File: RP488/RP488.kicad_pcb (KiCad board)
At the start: 2 copper layers, 56.1 x 53.1 mm, 25 parts, among them J1 GPIB, J2 Test, U1 SN75160, U2 SN75161, U3 SN74LV245ATDW

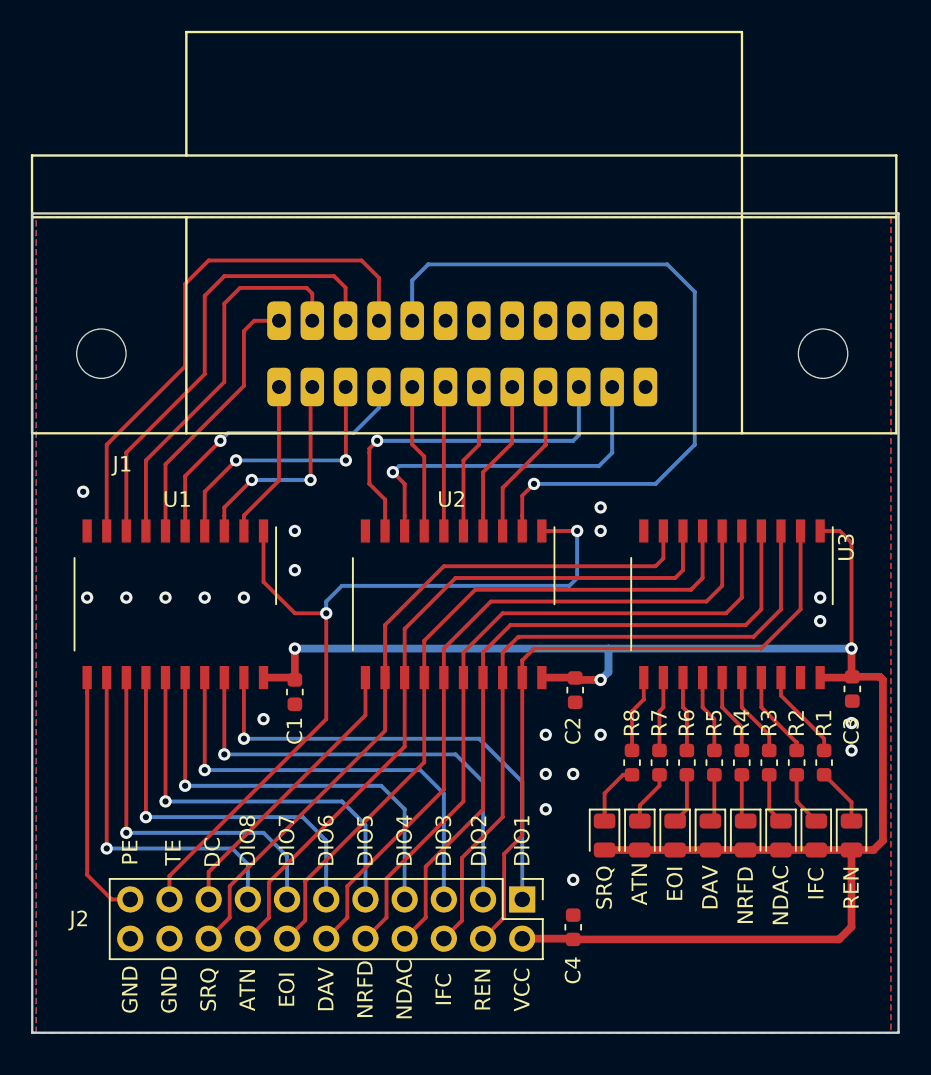
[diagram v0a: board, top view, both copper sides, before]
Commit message: SWD connector and schematic changes
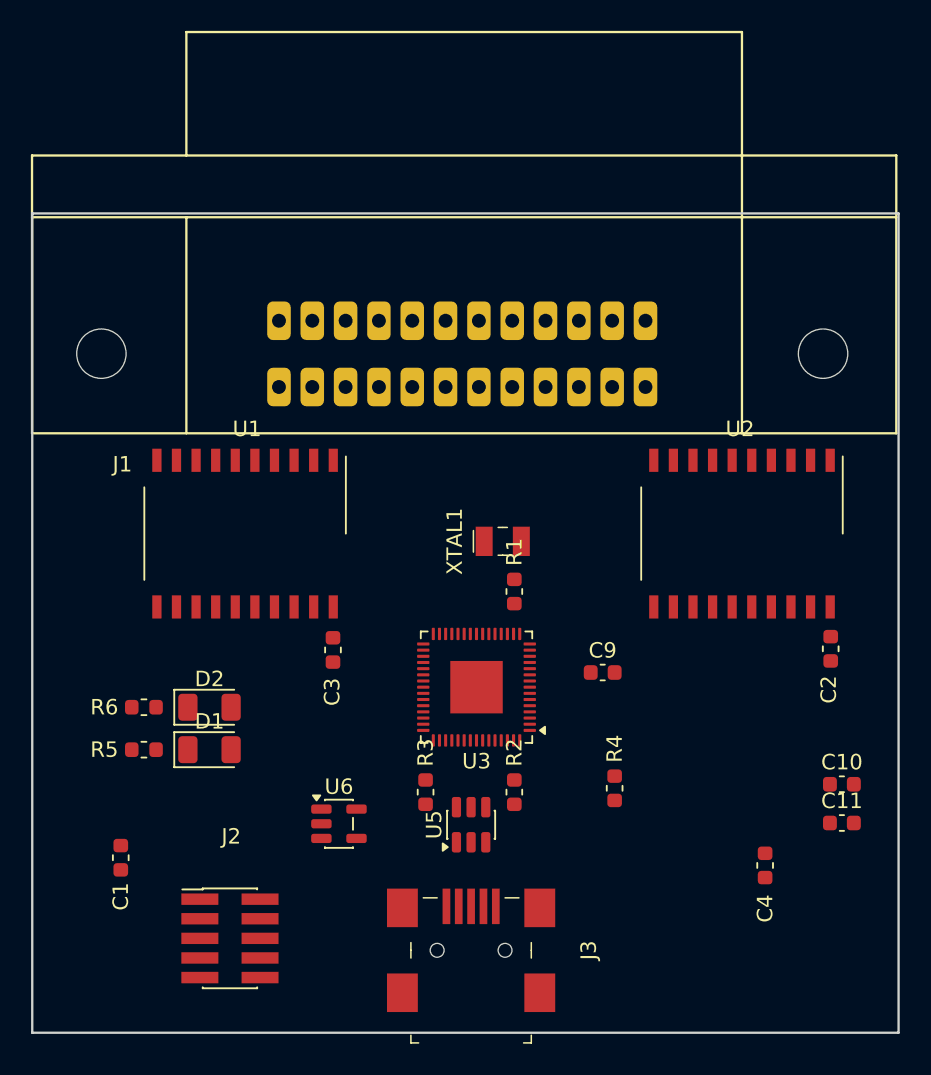
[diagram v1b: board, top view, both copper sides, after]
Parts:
- removed D3, D4, D5, D6, D7, D8: LED, LED_SMD:LED_0805_2012Metric
- removed R7, R8: 330R, Resistor_SMD:R_0603_1608Metric
- added C10: 100n, Capacitor_SMD:C_0603_1608Metric, F.Cu at (164.5, 100.7)
- added C11: 100n, Capacitor_SMD:C_0603_1608Metric, F.Cu at (164.5, 103.2)
- added C9: 100n, Capacitor_SMD:C_0603_1608Metric, F.Cu at (149.0, 93.5)
- added J3: USB Mini, GPIB:USB_Mini_B_Female_690-005-299-043, F.Cu at (140.4, 111.5)
- added U5: USBLC6-2SC6, Package_TO_SOT_SMD:SOT-23-6, F.Cu at (140.4, 103.4)
- added U6: LD3985M33R_SOT23, Package_TO_SOT_SMD:SOT-23-5, F.Cu at (131.9, 103.3)
- added XTAL1: 12MHz, GPIB:SMD-2_3.2x1.5mm, F.Cu at (142.5, 85.0)
- D1, D2: footprint LED_SMD:LED_0805_2012Metric -> LED_SMD:LED_1206_3216Metric
- J2: value Test -> SWD; footprint Connector_PinHeader_2.54mm:PinHeader_2x11_P2.54mm_Vertical -> GPIB:PinHeader_2x05_P1.27mm_Vertical_SMD
- R1, R5, R6: value 330R -> 1K
- R2, R3: value 330R -> 27R
- R4: value 330R -> 33R
- U3: value SN74LV245ATDW -> RP2354A; footprint Package_SO:SO-20_12.8x7.5mm_P1.27mm -> Package_DFN_QFN:QFN-60-1EP_7x7mm_P0.4mm_EP3.4x3.4mm
- moved D1 42.0 mm to (123.5, 98.5), turned to 0 degrees
- moved D2 40.2 mm to (123.5, 95.8), turned to 0 degrees
- moved R5 37.0 mm to (119.2, 98.5), turned to 180 degrees
- moved R6 35.4 mm to (119.2, 95.8), turned to 180 degrees
- moved C3 33.7 mm to (131.5, 92.0)
- moved R1 22.9 mm to (143.2, 88.2)
- moved R3 22.3 mm to (137.5, 101.2)
- moved U2 19.2 mm to (158.0, 84.5)
- moved J2 19.1 mm to (124.8, 110.7), turned to 0 degrees
- moved R2 18.4 mm to (143.2, 101.2)
- moved U3 17.4 mm to (140.8, 94.5), turned to 180 degrees
- moved C2 16.8 mm to (163.8, 92.0)
- moved C1 15.6 mm to (117.8, 105.5)
- moved C4 13.1 mm to (159.5, 106.0)
- moved R4 8.40 mm to (149.8, 101.0)
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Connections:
- D1 pad 1: Net-(D1-Pad1) -> Net-(D1-K)
- D1 pad 2: +5V -> Net-(D1-A)
- D2 pad 1: Net-(D2-Pad1) -> Net-(D2-K)
- D2 pad 2: +5V -> Net-(D2-A)
- J1 pad 12: Net-(J1-Pad12) -> unconnected-(J1-Pin_12-Pad12)
- J2 pad 1: Net-(J2-Pad1) -> +3V3
- J2 pad 10: Net-(J2-Pad10) -> /nRESET
- J2 pad 2: +5V -> /SWDIO
- J2 pad 3: Net-(J2-Pad3) -> GNDD
- J2 pad 4: Net-(J2-Pad4) -> /SWDCLK
- J2 pad 5: Net-(J2-Pad5) -> GNDD
- J2 pad 6: Net-(J2-Pad6) -> /SWO
- J2 pad 7: Net-(J2-Pad7) -> unconnected-(J2-Pin_7-Pad7)
- J2 pad 8: Net-(J2-Pad8) -> /TDI
- J2 pad 9: Net-(J2-Pad9) -> unconnected-(J2-Pin_9-Pad9)
- R1 pad 1: Net-(D1-Pad1) -> Net-(C5-Pad1)
- R1 pad 2: Net-(R1-Pad2) -> Net-(U3-XOUT)
- R2 pad 1: Net-(D2-Pad1) -> Net-(R2-Pad1)
- R2 pad 2: Net-(R2-Pad2) -> Net-(U3-USB_DP)
- R3 pad 2: Net-(R3-Pad2) -> Net-(U3-USB_DM)
- R4 pad 1: Net-(D4-Pad1) -> Net-(U3-VREG_AVDD)
- R4 pad 2: Net-(R4-Pad2) -> +3V3
- R5 pad 1: Net-(D5-Pad1) -> Net-(D1-K)
- R5 pad 2: Net-(R5-Pad2) -> GNDD
- R6 pad 1: Net-(D6-Pad1) -> Net-(D2-K)
- R6 pad 2: Net-(R6-Pad2) -> GNDD
- U1 pad 1: Net-(J2-Pad19) -> Net-(U1-TE)
- U1 pad 11: Net-(J2-Pad21) -> Net-(U1-PE)
- U1 pad 12: Net-(J2-Pad15) -> Net-(U1-D8)
- U1 pad 13: Net-(J2-Pad13) -> Net-(U1-D7)
- U1 pad 14: Net-(J2-Pad11) -> Net-(U1-D6)
- U1 pad 15: Net-(J2-Pad9) -> Net-(U1-D5)
- U1 pad 16: Net-(J2-Pad7) -> Net-(U1-D4)
- U1 pad 17: Net-(J2-Pad5) -> Net-(U1-D3)
- U1 pad 18: Net-(J2-Pad3) -> Net-(U1-D2)
- U1 pad 19: Net-(J2-Pad1) -> Net-(U1-D1)
- U1 pad 9: /DIO8 -> unconnected-(U1-B8-Pad9)
- U2 pad 1: Net-(J2-Pad19) -> Net-(U1-TE)
- U2 pad 11: Net-(J2-Pad17) -> Net-(U2-DC)
- U2 pad 12: Net-(J2-Pad18) -> Net-(U3-GPIO13)
- U2 pad 13: Net-(J2-Pad16) -> Net-(U3-GPIO12)
- U2 pad 14: Net-(J2-Pad14) -> Net-(U3-GPIO11)
- U2 pad 15: Net-(J2-Pad12) -> Net-(U3-GPIO8)
- U2 pad 16: Net-(J2-Pad10) -> Net-(U3-GPIO9)
- U2 pad 17: Net-(J2-Pad8) -> Net-(U3-GPIO10)
- U2 pad 18: Net-(J2-Pad6) -> Net-(U3-GPIO14)
- U2 pad 19: Net-(J2-Pad4) -> Net-(U3-GPIO15)
- U3 pad 1: +5V -> +3V3
- U3 pad 10: GNDD -> Net-(U1-D8)
- U3 pad 11: Net-(R8-Pad2) -> +3V3
- U3 pad 12: Net-(R7-Pad2) -> Net-(U3-GPIO8)
- U3 pad 13: Net-(R6-Pad2) -> Net-(U3-GPIO9)
- U3 pad 14: Net-(R5-Pad2) -> Net-(U3-GPIO10)
- U3 pad 15: Net-(R4-Pad2) -> Net-(U3-GPIO11)
- U3 pad 16: Net-(R3-Pad2) -> Net-(U3-GPIO12)
- U3 pad 17: Net-(R2-Pad2) -> Net-(U3-GPIO13)
- U3 pad 18: Net-(R1-Pad2) -> Net-(U3-GPIO14)
- U3 pad 19: GNDD -> Net-(U3-GPIO15)
- U3 pad 2: Net-(J2-Pad4) -> Net-(U1-D1)
- U3 pad 20: +5V -> +3V3
- U3 pad 3: Net-(J2-Pad6) -> Net-(U1-D2)
- U3 pad 4: Net-(J2-Pad8) -> Net-(U1-D3)
- U3 pad 5: Net-(J2-Pad10) -> Net-(U1-D4)
- U3 pad 6: Net-(J2-Pad12) -> Net-(U3-VREG_FB)
- U3 pad 7: Net-(J2-Pad14) -> Net-(U1-D5)
- U3 pad 8: Net-(J2-Pad16) -> Net-(U1-D6)
- U3 pad 9: Net-(J2-Pad18) -> Net-(U1-D7)
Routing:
- net +5V: track 116.9 -> 0.00 mm, vias 3 -> 0
- net Net-(J2-Pad19): track 53.9 -> 0.00 mm, vias 2 -> 0
- net /REN: track 46.8 -> 0.00 mm, vias 1 -> 0
- net Net-(J2-Pad18): track 46.7 -> 0.00 mm
- net Net-(J2-Pad16): track 46.4 -> 0.00 mm
- net Net-(J2-Pad14): track 45.8 -> 0.00 mm
- net Net-(J2-Pad12): track 45.2 -> 0.00 mm
- net Net-(J2-Pad10): track 45.0 -> 0.00 mm
- net Net-(J2-Pad8): track 44.9 -> 0.00 mm
- net Net-(J2-Pad6): track 44.4 -> 0.00 mm
- net Net-(J2-Pad4): track 43.6 -> 0.00 mm
- net /DIO8: track 34.5 -> 0.00 mm
- net Net-(J2-Pad1): track 30.8 -> 0.00 mm, vias 1 -> 0
- net Net-(J2-Pad3): track 30.1 -> 0.00 mm, vias 1 -> 0
- net /DIO7: track 29.5 -> 0.00 mm
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- removed copper zone on B.Cu, net GNDD
- removed copper zone on F.Cu, net GNDD
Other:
- board text removed: "ATN"
- board text removed: "DAV"
- board text removed: "DC"
- board text removed: "DIO1"
- board text removed: "DIO2"
- board text removed: "DIO3"
- board text removed: "DIO4"
- board text removed: "DIO5"
- board text removed: "DIO6"
- board text removed: "DIO7"
- board text removed: "DIO8"
- board text removed: "EOI"
- board text removed: "GND"
- board text removed: "IFC"
- board text removed: "NDAC"
- board text removed: "NRFD"
- board text removed: "PE"
- board text removed: "REN"
- board text removed: "SRQ"
- board text removed: "TE"
- board text removed: "VCC"

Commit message: Switch to RP2354
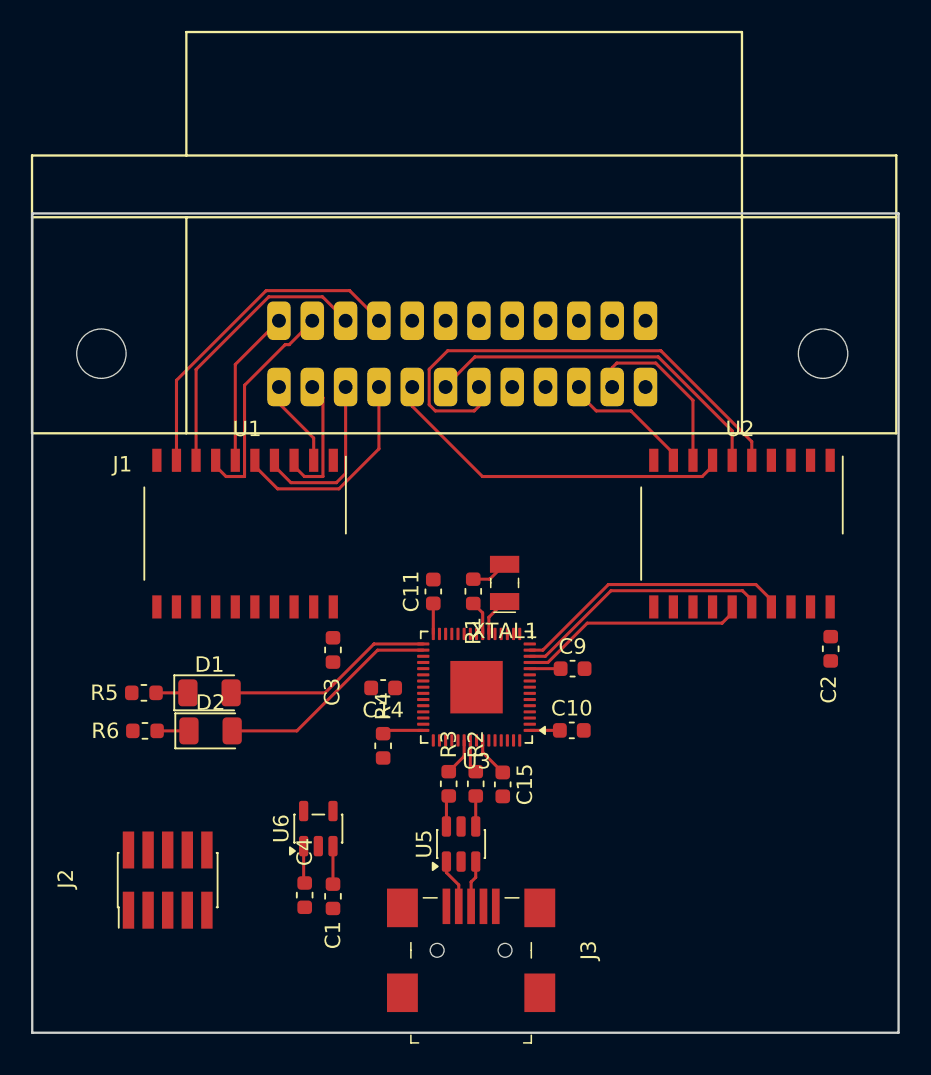
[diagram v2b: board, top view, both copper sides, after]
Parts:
- added C14: 100n, Capacitor_SMD:C_0603_1608Metric, F.Cu at (134.8, 94.5)
- added C15: 100n, Capacitor_SMD:C_0603_1608Metric, F.Cu at (142.5, 100.8)
- moved C11 30.4 mm to (138.0, 88.2), turned to 90 degrees
- moved C4 29.9 mm to (129.7, 107.9), turned to -90 degrees
- moved C10 17.8 mm to (147.0, 97.2)
- moved R4 15.2 mm to (134.8, 98.2)
- moved C1 14.0 mm to (131.5, 108.0)
- moved J2 5.53 mm to (120.8, 107.0), turned to 90 degrees
- moved D1 3.68 mm to (123.5, 94.8)
- moved R5 3.68 mm to (119.2, 94.8)
- moved XTAL1 2.70 mm to (142.6, 87.7), turned to 90 degrees
- moved R1 2.66 mm to (140.6, 88.2), turned to -90 degrees
- moved R2 2.56 mm to (140.8, 100.7)
- moved C9 1.97 mm to (147.0, 93.2)
- moved R3 1.59 mm to (139.0, 100.7)
- moved D2 1.53 mm to (123.6, 97.3)
- moved R6 1.53 mm to (119.3, 97.3)
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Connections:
- U1 pad 9: unconnected-(U1-B8-Pad9) -> /DIO8
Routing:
- net /NRFD: track 0.00 -> 32.1 mm
- net /DAV: track 0.00 -> 23.3 mm
- net /EOI: track 0.00 -> 23.3 mm
- net /DIO8: track 0.00 -> 21.5 mm
- net Net-(U3-GPIO10): track 0.00 -> 18.3 mm
- net /DIO7: track 0.00 -> 18.2 mm
- net Net-(U3-GPIO9): track 0.00 -> 16.8 mm
- net Net-(U3-GPIO8): track 0.00 -> 14.8 mm
- net /DIO6: track 0.00 -> 14.6 mm
- net Net-(D2-A): track 0.00 -> 14.5 mm
- net /DIO4: track 0.00 -> 14.1 mm
- net Net-(D1-A): track 0.00 -> 13.8 mm
- net /ATN: track 0.00 -> 11.5 mm
- net /DIO3: track 0.00 -> 11.3 mm
- net +3V3: track 0.00 -> 11.2 mm
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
